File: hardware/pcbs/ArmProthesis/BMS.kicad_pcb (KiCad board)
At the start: 4 copper layers, 96.9 x 57 mm, 58 parts, among them J1 XT60-M, J2 XT60-F, J3 4-1971800-1, Q1 BSC014N04LSIATMA1, Q2 BSC014N04LSIATMA1, Q3 BSS84, SW1 CK_KMS2xxG, SW2 CK_KMS2xxG, SW3 CK_KMS2xxG, SW4 CK_KMS2xxG, U1 BQ76920PW, U6 STM32C011F6Px, Y1 Crystal

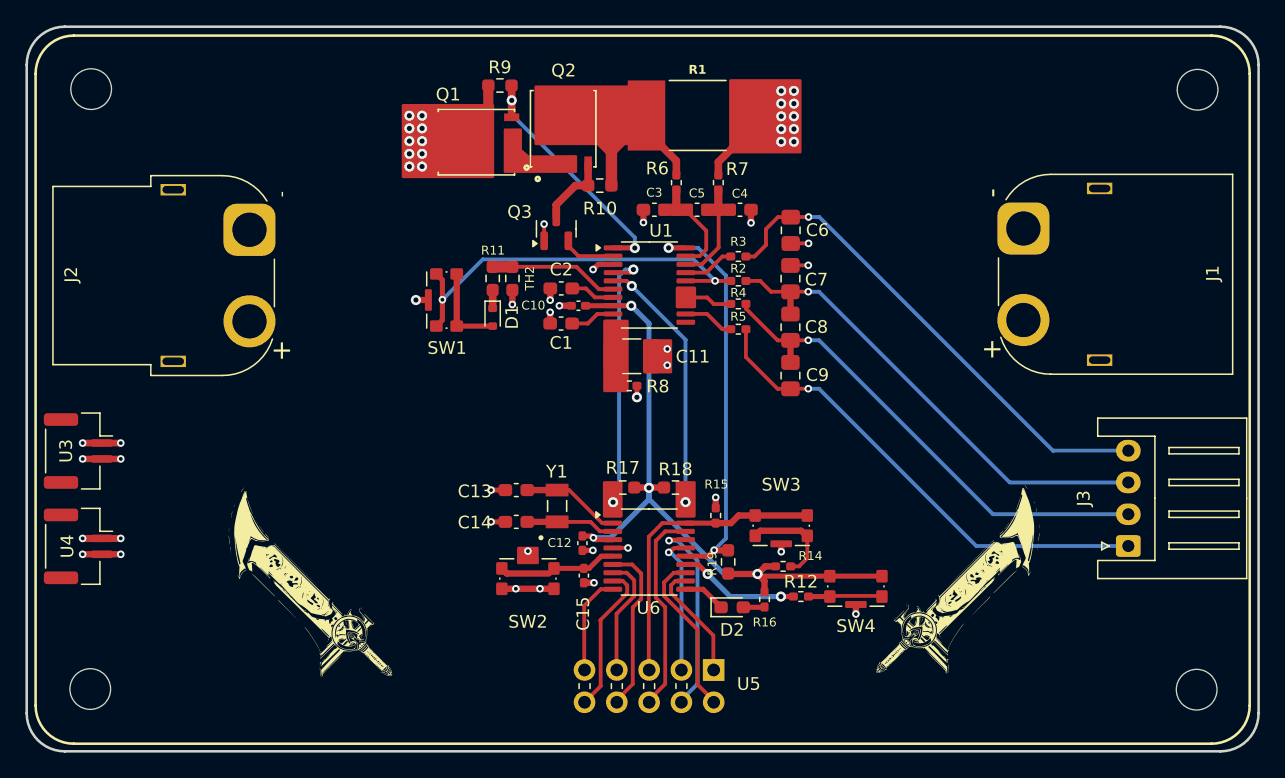
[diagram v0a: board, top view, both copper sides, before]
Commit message: .
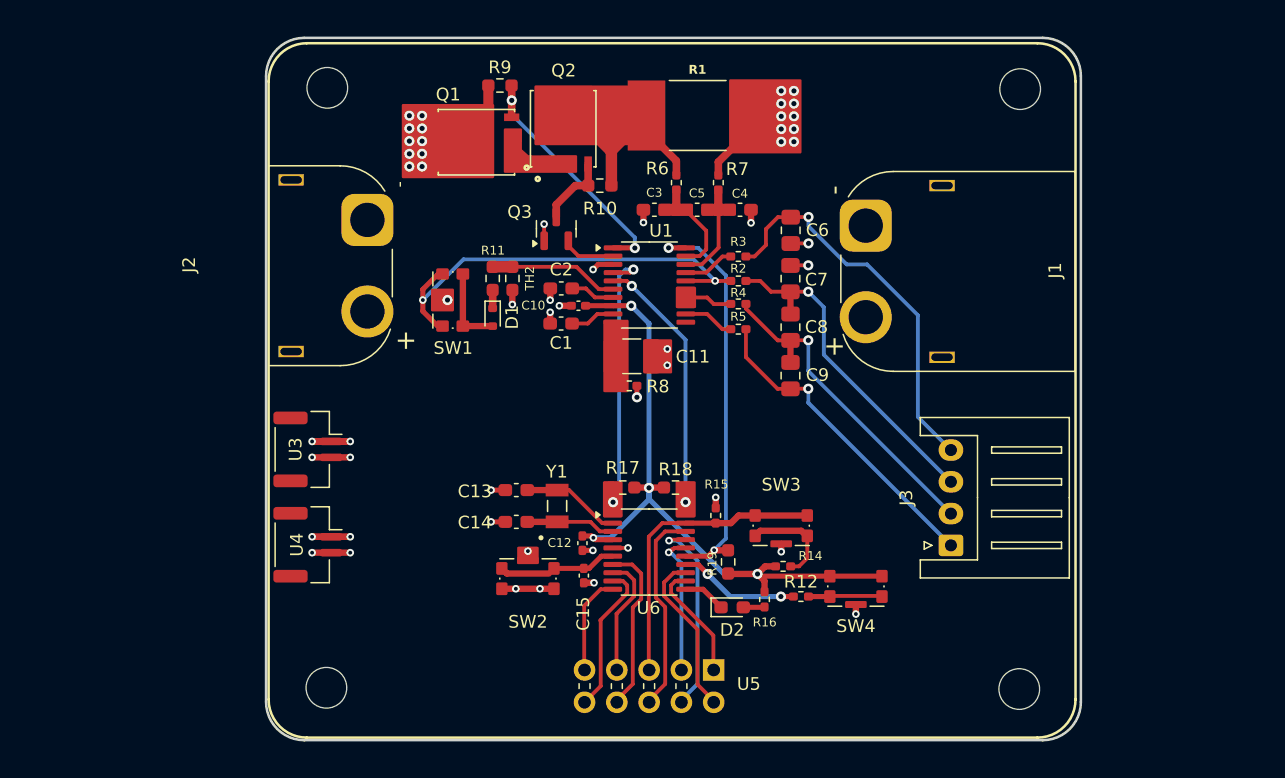
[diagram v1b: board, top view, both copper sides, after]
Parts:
- removed G***: LOGO, Pics:riven_sword_20mm_quality
- removed REF**: riven_sword_20mm_quality_mirrored, Pics:riven_sword_20mm_quality_mirrored
- moved H1 18.6 mm to (126.5, 78.5)
- moved H3 18.6 mm to (126.5, 125.7)
- moved U3 18.1 mm to (125.0, 107.0)
- moved U4 18.1 mm to (125.0, 114.5)
- moved H2 14.0 mm to (181.0, 78.6)
- moved H4 14.0 mm to (181.0, 125.8)
- moved J3 14.0 mm to (175.6, 114.5)
- moved J1 12.4 mm to (168.9, 89.3)
- moved J2 9.31 mm to (129.7, 88.9)
- moved SW1 0.48 mm to (136.4, 95.2)
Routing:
- net Net-(C9-Pad1): track 38.4 -> 25.1 mm
- net Net-(C8-Pad1): track 39.0 -> 26.4 mm
- net Net-(C7-Pad1): track 38.4 -> 26.6 mm
- net Net-(C6-Pad2): track 39.7 -> 30.9 mm
- net Net-(U1-VC1): track 31.5 -> 34.6 mm
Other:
- board size 96.9 x 57 mm -> 64.1 x 55.2 mm
